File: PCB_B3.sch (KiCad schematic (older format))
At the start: 18 parts, among them J1 Screw_Terminal_01x02, J2 Screw_Terminal_01x02, J3 Conn_01x03_Male, J4 Conn_01x03_Male, J5 Conn_01x04_Male, K1 G3MB202PDC12, P1 Digital, P3 ADC, P4 Analog, P5 ADC, U2 BC547C, U3 NRF24L01_Breakout

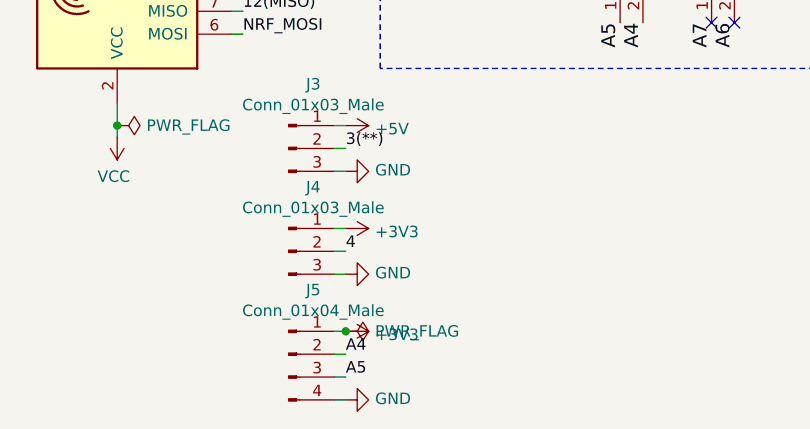
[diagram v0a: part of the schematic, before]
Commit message: Update
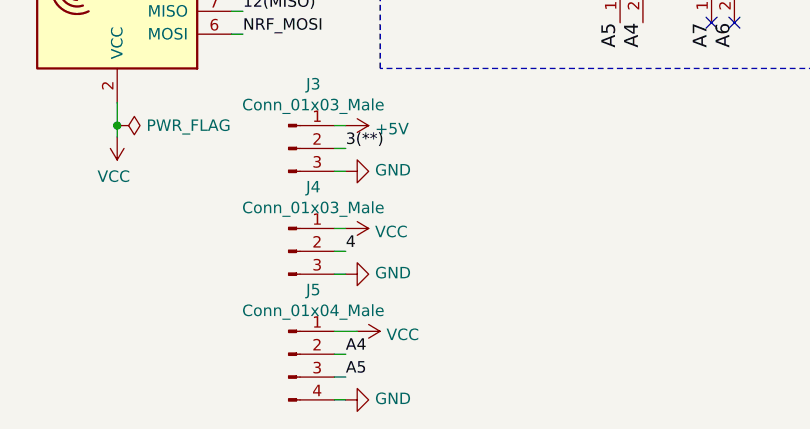
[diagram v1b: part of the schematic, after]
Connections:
- net labels removed: +3V3
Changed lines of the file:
@@
-	0    1    1    0
-$EndComp
-$Comp
-L power:+3V3 #PWR012
-U 1 1 60101D38
-P 8350 4100
-F 0 "#PWR012" H 8350 3950 50  0001 C CNN
-F 1 "+3V3" V 8365 4228 50  0000 L CNN
-F 2 "" H 8350 4100 50  0001 C CNN
-F 3 "" H 8350 4100 50  0001 C CNN
-	1    8350 4100
 	0    1    1    0
 $EndComp
@@
 Wire Wire Line
 	7000 875  7000 900
-Connection ~ 8350 4550
-Wire Wire Line
-	8300 4550 8350 4550
-$Comp
-L power:+3V3 #PWR014
-U 1 1 60109C1C
-P 8350 4550
-F 0 "#PWR014" H 8350 4400 50  0001 C CNN
-F 1 "+3V3" V 8365 4678 50  0000 L CNN
-F 2 "" H 8350 4550 50  0001 C CNN
-F 3 "" H 8350 4550 50  0001 C CNN
-	1    8350 4550
-	0    1    1    0
-$EndComp
-$Comp
-L power:PWR_FLAG #FLG0102
-U 1 1 601A1D5A
-P 8350 4550
-F 0 "#FLG0102" H 8350 4625 50  0001 C CNN
-F 1 "PWR_FLAG" V 8350 4678 50  0000 L CNN
-F 2 "" H 8350 4550 50  0001 C CNN
-F 3 "~" H 8350 4550 50  0001 C CNN
-	1    8350 4550
-	0    1    1    0
-$EndComp
 Wire Wire Line
 	6350 800  6350 875
@@
 	1    0    0    -1
 $EndComp
+$Comp
+L power:VCC #PWR?
+U 1 1 6022B4A2
+P 8350 4100
+F 0 "#PWR?" H 8350 3950 50  0001 C CNN
+F 1 "VCC" V 8365 4228 50  0000 L CNN
+F 2 "" H 8350 4100 50  0001 C CNN
+F 3 "" H 8350 4100 50  0001 C CNN
+	1    8350 4100
+	0    1    1    0
+$EndComp
+$Comp
+L power:VCC #PWR?
+U 1 1 6022C566
+P 8400 4550
+F 0 "#PWR?" H 8400 4400 50  0001 C CNN
+F 1 "VCC" V 8415 4678 50  0000 L CNN
+F 2 "" H 8400 4550 50  0001 C CNN
+F 3 "" H 8400 4550 50  0001 C CNN
+	1    8400 4550
+	0    1    1    0
+$EndComp
+Wire Wire Line
+	8300 4550 8400 4550
 $EndSCHEMATC
